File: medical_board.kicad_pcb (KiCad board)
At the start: 2 copper layers, 115.3 x 47.2 mm, 72 parts, among them M1 JST_XH_S2B-XH-A-1_1x02_P2.50m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, M2 JST_XH_S2B-XH-A-1_1x02_P2.50m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, M3 JST_XH_S2B-XH-A-1_1x02_P2.50m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, M4 JST_XH_S2B-XH-A-1_1x02_P2.50m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, M5 JST_XH_S2B-XH-A-1_1x02_P2.50m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, U1 OPAMP, U2 OPAMP, U3 OPAMP, U4 OPAMP, U5 OPAMP, U6 OPAMP

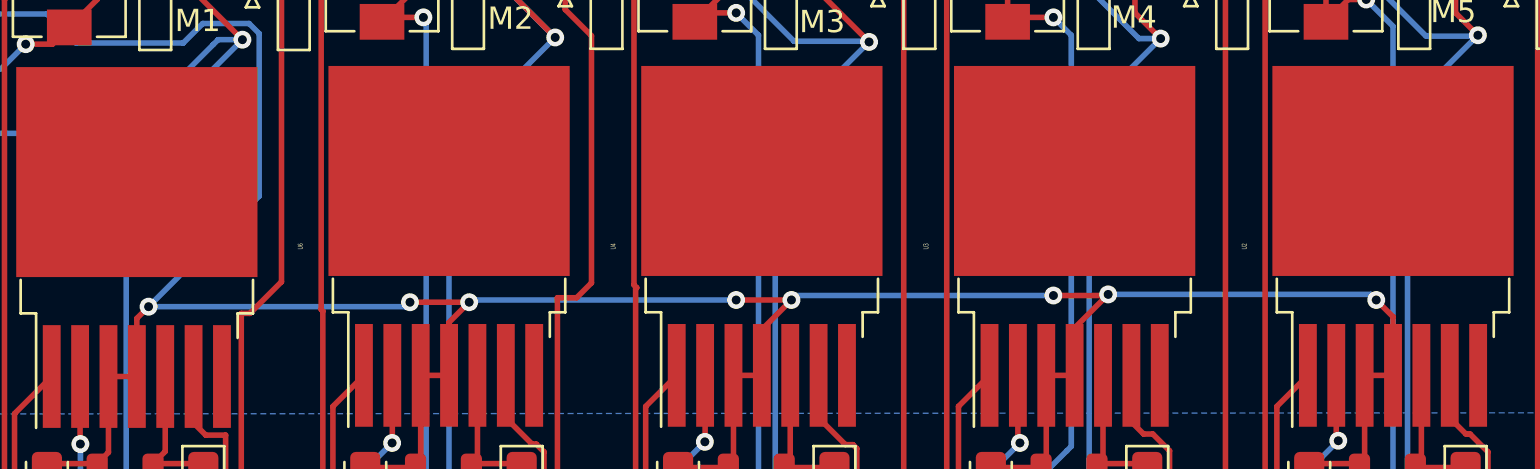
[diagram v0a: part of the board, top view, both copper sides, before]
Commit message: Updated Routing files
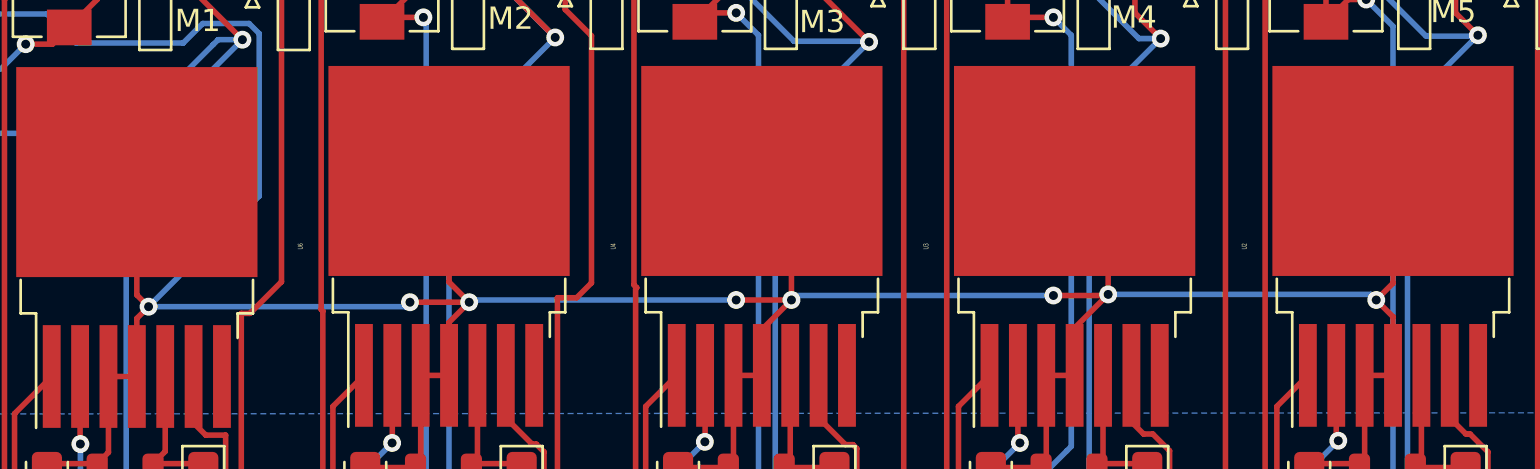
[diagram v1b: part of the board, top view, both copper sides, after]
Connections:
- U2 pad 8: (no net) -> -V
- U3 pad 8: (no net) -> -V
- U4 pad 8: (no net) -> -V
- U5 pad 8: (no net) -> -V
- U6 pad 8: (no net) -> -V
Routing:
- net -V: track 305.8 -> 336.9 mm
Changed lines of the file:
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@@
       (net 8 "Net-(D11-Pad2)"))
     (pad "7" smd rect (at -5.775 3.81 90) (size 4.6 0.8) (layers "F.Cu" "F.Paste" "F.Mask"))
-    (pad "8" smd rect (at 3.375 0 90) (size 9.4 10.8) (layers "F.Cu" "F.Mask"))
+    (pad "8" smd rect (at 3.375 0 90) (size 9.4 10.8) (layers "F.Cu" "F.Mask")
+      (net 3 "-V"))
     (model "${KICAD6_3DMODEL_DIR}/Package_TO_SOT_SMD.3dshapes/TO-263-7_TabPin8.wrl"
       (offset (xyz 0 0 0))
@@
       (net 5 "Net-(D5-Pad2)"))
     (pad "7" smd rect (at -5.775 3.81 90) (size 4.6 0.8) (layers "F.Cu" "F.Paste" "F.Mask"))
-    (pad "8" smd rect (at 3.375 0 90) (size 9.4 10.8) (layers "F.Cu" "F.Mask"))
+    (pad "8" smd rect (at 3.375 0 90) (size 9.4 10.8) (layers "F.Cu" "F.Mask")
+      (net 3 "-V"))
     (model "${KICAD6_3DMODEL_DIR}/Package_TO_SOT_SMD.3dshapes/TO-263-7_TabPin8.wrl"
       (offset (xyz 0 0 0))
@@
       (net 4 "Net-(D3-Pad2)"))
     (pad "7" smd rect (at -5.775 3.81 90) (size 4.6 0.8) (layers "F.Cu" "F.Paste" "F.Mask"))
-    (pad "8" smd rect (at 3.375 0 90) (size 9.4 10.8) (layers "F.Cu" "F.Mask"))
+    (pad "8" smd rect (at 3.375 0 90) (size 9.4 10.8) (layers "F.Cu" "F.Mask")
+      (net 3 "-V"))
     (model "${KICAD6_3DMODEL_DIR}/Package_TO_SOT_SMD.3dshapes/TO-263-7_TabPin8.wrl"
       (offset (xyz 0 0 0))
@@
       (net 6 "Net-(D7-Pad2)"))
     (pad "7" smd rect (at -5.775 3.81 90) (size 4.6 0.8) (layers "F.Cu" "F.Paste" "F.Mask"))
-    (pad "8" smd rect (at 3.375 0 90) (size 9.4 10.8) (layers "F.Cu" "F.Mask"))
+    (pad "8" smd rect (at 3.375 0 90) (size 9.4 10.8) (layers "F.Cu" "F.Mask")
+      (net 3 "-V"))
     (model "${KICAD6_3DMODEL_DIR}/Package_TO_SOT_SMD.3dshapes/TO-263-7_TabPin8.wrl"
       (offset (xyz 0 0 0))
@@
       (net 7 "Net-(D10-Pad1)"))
     (pad "7" smd rect (at -5.775 3.81 90) (size 4.6 0.8) (layers "F.Cu" "F.Paste" "F.Mask"))
-    (pad "8" smd rect (at 3.375 0 90) (size 9.4 10.8) (layers "F.Cu" "F.Mask"))
+    (pad "8" smd rect (at 3.375 0 90) (size 9.4 10.8) (layers "F.Cu" "F.Mask")
+      (net 3 "-V"))
     (model "${KICAD6_3DMODEL_DIR}/Package_TO_SOT_SMD.3dshapes/TO-263-7_TabPin8.wrl"
       (offset (xyz 0 0 0))
@@
   (segment (start 139.6 92.9) (end 138.28 92.9) (width 0.25) (layer "B.Cu") (net 2))
   (segment (start 164.524511 93.362989) (end 164.524511 71.924511) (width 0.25) (layer "B.Cu") (net 2))
+  (segment (start 166.45 84.55) (end 165.55 83.65) (width 0.25) (layer "F.Cu") (net 3))
   (segment (start 137.65371 69.04629) (end 139.2 67.5) (width 1.00838) (layer "F.Cu") (net 3))
   (segment (start 178.4 84.45) (end 180.8745 84.45) (width 0.25) (layer "F.Cu") (net 3))
@@
   (segment (start 122.3 69.35) (end 117.65 69.35) (width 0.25) (layer "F.Cu") (net 3))
   (segment (start 164.28 87.825) (end 165.55 87.825) (width 0.25) (layer "F.Cu") (net 3))
+  (segment (start 151.575 84.225) (end 151.575 78.725) (width 0.25) (layer "F.Cu") (net 3))
   (segment (start 112.95 72.35) (end 114.65 72.35) (width 0.25) (layer "F.Cu") (net 3))
   (segment (start 164.28 87.825) (end 164.28 91.545) (width 0.25) (layer "F.Cu") (net 3))
@@
   (segment (start 193.55 87.825) (end 193.55 85.7) (width 0.25) (layer "F.Cu") (net 3))
   (segment (start 203.05048 92.94952) (end 204.05 91.95) (width 0.25) (layer "F.Cu") (net 3))
+  (segment (start 195.05 84.2) (end 195.05 80.175) (width 0.25) (layer "F.Cu") (net 3))
   (segment (start 177.15 97.8) (end 174.80048 95.45048) (width 0.25) (layer "F.Cu") (net 3))
   (segment (start 175.8 91.95) (end 177.875 91.95) (width 0.25) (layer "F.Cu") (net 3))
@@
   (segment (start 206.53 91.545) (end 206.3 91.775) (width 0.25) (layer "F.Cu") (net 3))
   (segment (start 174.80048 92.94952) (end 175.8 91.95) (width 0.25) (layer "F.Cu") (net 3))
+  (segment (start 180.8745 79.9995) (end 179.55 78.675) (width 0.25) (layer "F.Cu") (net 3))
   (segment (start 126.65 70.85) (end 129.8 67.7) (width 1.00838) (layer "F.Cu") (net 3))
   (segment (start 160.80048 95.45048) (end 163.15 97.8) (width 0.25) (layer "F.Cu") (net 3))
   (segment (start 124.2 102.3) (end 124.2 101.1) (width 1.00838) (layer "F.Cu") (net 3))
   (segment (start 150.305 91.27) (end 149.8 91.775) (width 0.25) (layer "F.Cu") (net 3))
+  (segment (start 207.8 83.7) (end 207.8 78.675) (width 0.25) (layer "F.Cu") (net 3))
+  (segment (start 195.05 80.175) (end 193.55 78.675) (width 0.25) (layer "F.Cu") (net 3))
   (segment (start 151.575 85.275) (end 152.1 84.75) (width 0.25) (layer "F.Cu") (net 3))
   (segment (start 163.8 84.55) (end 166.45 84.55) (width 0.25) (layer "F.Cu") (net 3))
   (segment (start 160.80048 92.94952) (end 160.80048 95.45048) (width 0.25) (layer "F.Cu") (net 3))
+  (segment (start 180.8745 84.45) (end 180.8745 79.9995) (width 0.25) (layer "F.Cu") (net 3))
   (segment (start 207.8 85.2) (end 207.05 84.45) (width 0.25) (layer "F.Cu") (net 3))
   (segment (start 143.9 68.85) (end 143.9 68.3) (width 0.25) (layer "F.Cu") (net 3))
@@
   (segment (start 131.575 102.8) (end 131.575 100.875) (width 1.00838) (layer "F.Cu") (net 3))
   (segment (start 143.9 68.3) (end 141.9 66.3) (width 0.25) (layer "F.Cu") (net 3))
+  (segment (start 165.55 83.65) (end 165.55 78.675) (width 0.25) (layer "F.Cu") (net 3))
   (segment (start 141.9 66.3) (end 125.35 66.3) (width 0.25) (layer "F.Cu") (net 3))
   (segment (start 135.375 69.8) (end 136.12871 69.04629) (width 1.00838) (layer "F.Cu") (net 3))
@@
   (segment (start 192.6 84.25) (end 195 84.25) (width 0.25) (layer "F.Cu") (net 3))
   (segment (start 193.55 87.825) (end 192.28 87.825) (width 0.25) (layer "F.Cu") (net 3))
+  (segment (start 207.8 78.675) (end 207.875 78.675) (width 1.00838) (layer "F.Cu") (net 3))
   (segment (start 207.8 87.825) (end 207.8 85.2) (width 0.25) (layer "F.Cu") (net 3))
+  (segment (start 207.05 84.45) (end 207.8 83.7) (width 0.25) (layer "F.Cu") (net 3))
   (segment (start 165.55 87.825) (end 165.55 85.45) (width 0.25) (layer "F.Cu") (net 3))
+  (segment (start 152.1 84.75) (end 151.575 84.225) (width 0.25) (layer "F.Cu") (net 3))
   (segment (start 195 84.25) (end 195.05 84.2) (width 0.25) (layer "F.Cu") (net 3))
   (segment (start 178.28 91.545) (end 178.05 91.775) (width 0.25) (layer "F.Cu") (net 3))
